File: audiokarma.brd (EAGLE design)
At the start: 72.3 x 42.2 mm, 63 parts, among them IC1 OPA2134U, IC2 OPA2134U

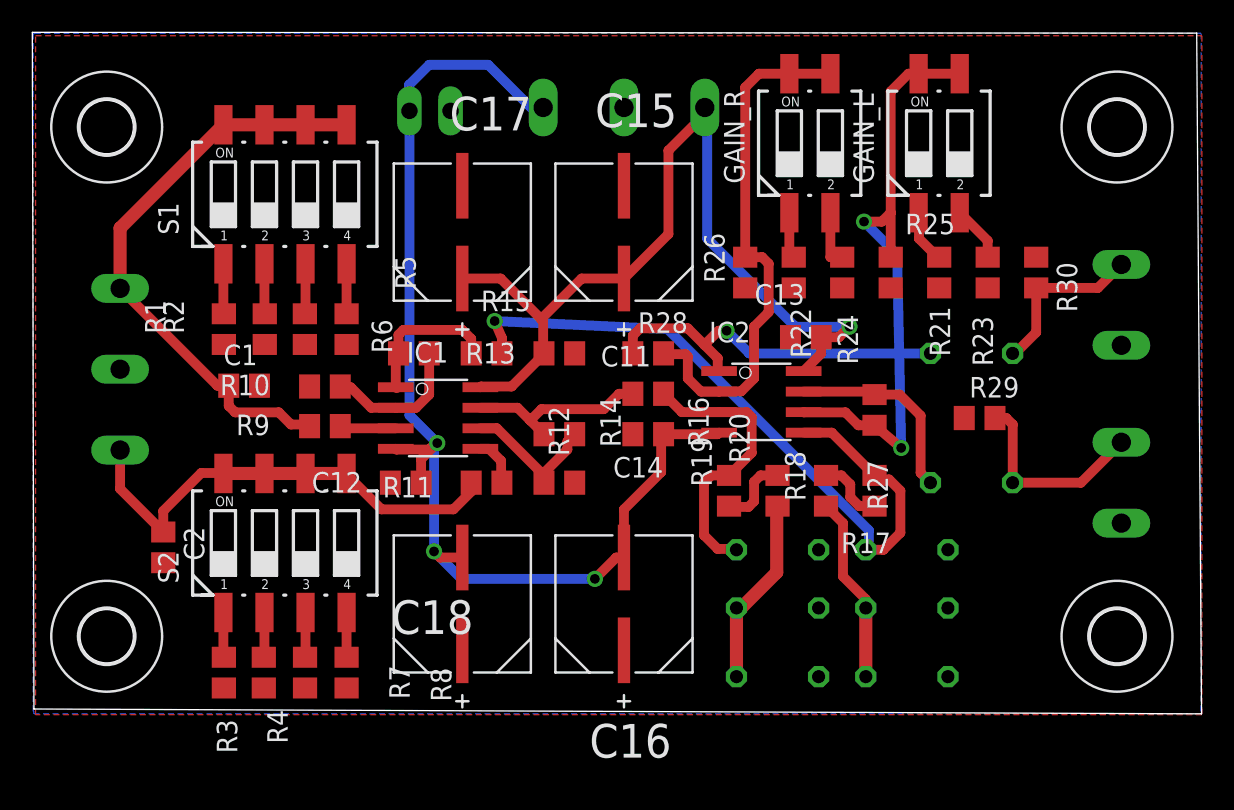
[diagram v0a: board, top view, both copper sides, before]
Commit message: Phono100% e inicio de supply
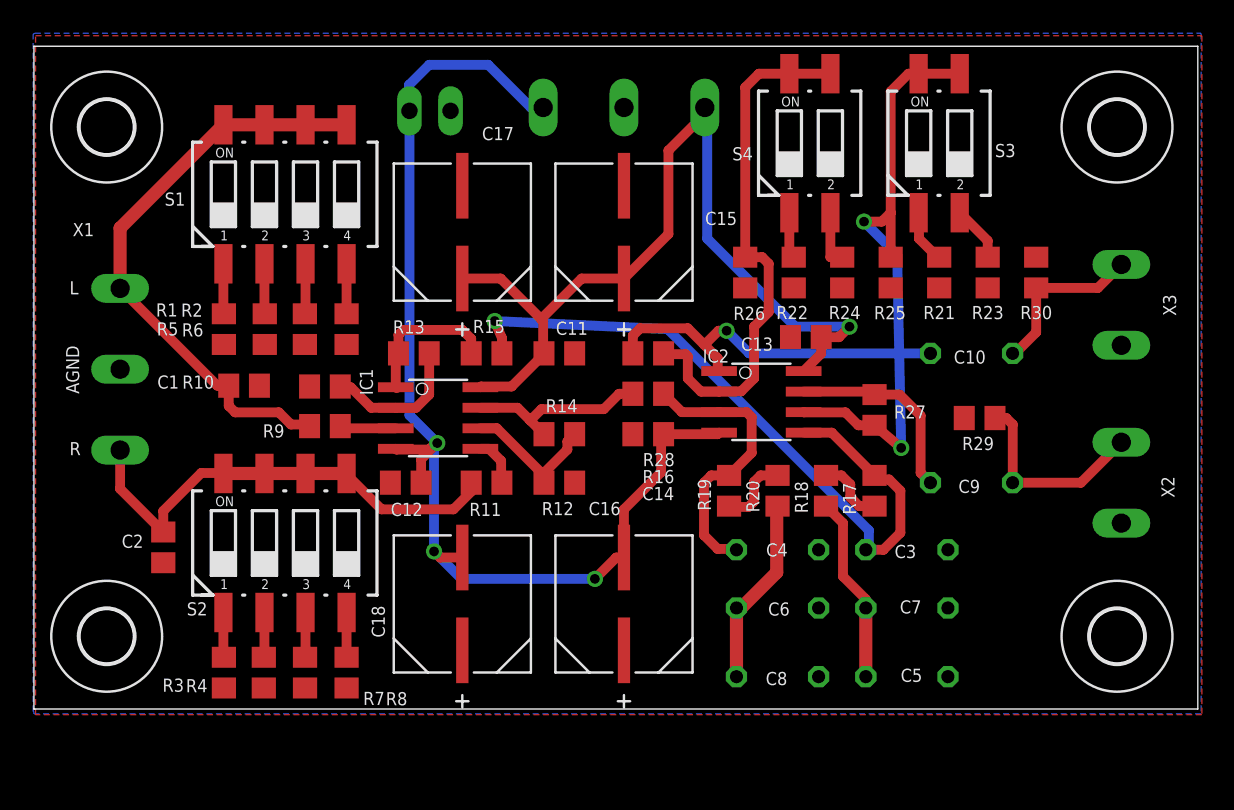
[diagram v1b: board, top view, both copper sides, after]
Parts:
- renumbered GAIN_L to S3, GAIN_R to S4
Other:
- board size 72.3 x 42.2 mm -> 72 x 41 mm
- board text added: "AGND"
- board text added: "L"
- board text added: "R"
